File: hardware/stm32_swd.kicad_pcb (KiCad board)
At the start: 2 copper layers, 35 parts, among them J5 SWD_SWD, J6 SWD_SWD, U6 STM32F103C8T6_rect, U7 SWD, U8 AMS1117-3.3, U9 USBLC6-2SC6_SOT23-6, Y1 O_8M

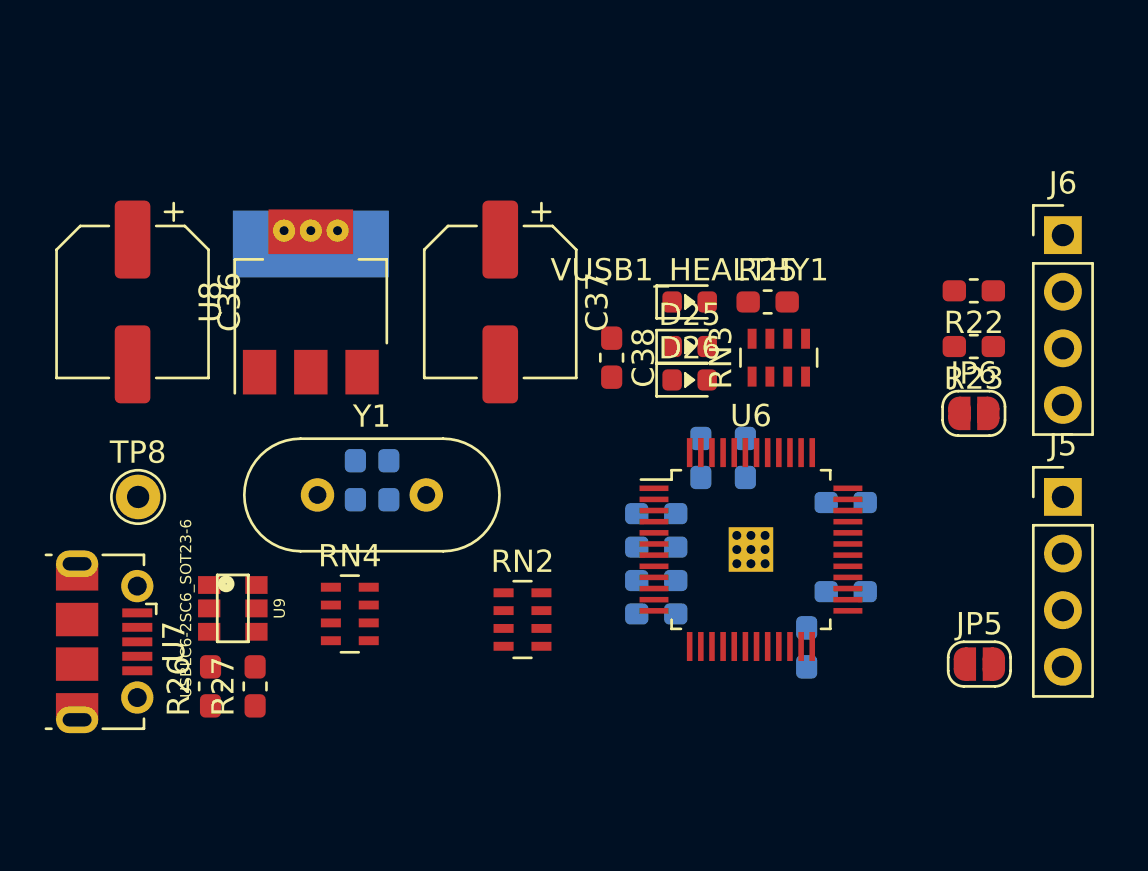
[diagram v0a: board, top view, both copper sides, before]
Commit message: update route,
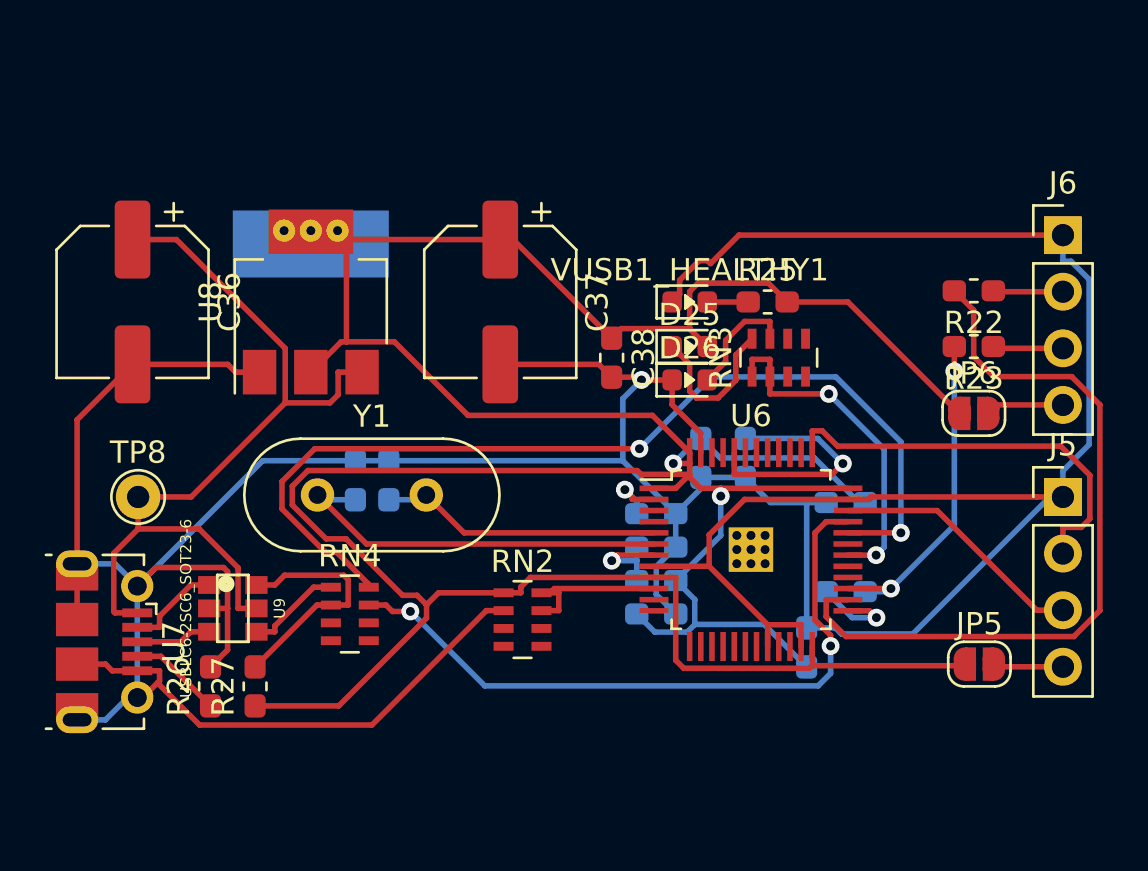
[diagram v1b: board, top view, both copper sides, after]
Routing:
- net GND: track 0.00 -> 200.6 mm, vias 0 -> 1
- net Vstm32_stlink: track 0.00 -> 166.6 mm, vias 0 -> 2
- net /USB_N: track 0.00 -> 44.0 mm, vias 0 -> 2
- net Vusb_1: track 0.00 -> 38.8 mm
- net /T_JTCK: track 0.00 -> 34.0 mm
- net /USB_P: track 0.00 -> 30.7 mm, vias 0 -> 2
- net /SWCLK: track 0.00 -> 18.8 mm
- net Net-(C29-Pad2): track 0.00 -> 17.8 mm
- net /LED_STLINK: track 0.00 -> 15.4 mm, vias 0 -> 2
- net /T_JTMS: track 0.00 -> 15.2 mm, vias 0 -> 2
- net Net-(C30-Pad2): track 0.00 -> 12.7 mm
- net /SWDIO: track 0.00 -> 11.5 mm
- net Net-(R20-Pad2): track 0.00 -> 10.9 mm, vias 0 -> 1
- net Net-(R27-Pad2): track 0.00 -> 10.8 mm
- net Net-(RN2-Pad7): track 0.00 -> 7.09 mm
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
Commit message: update ws2812,
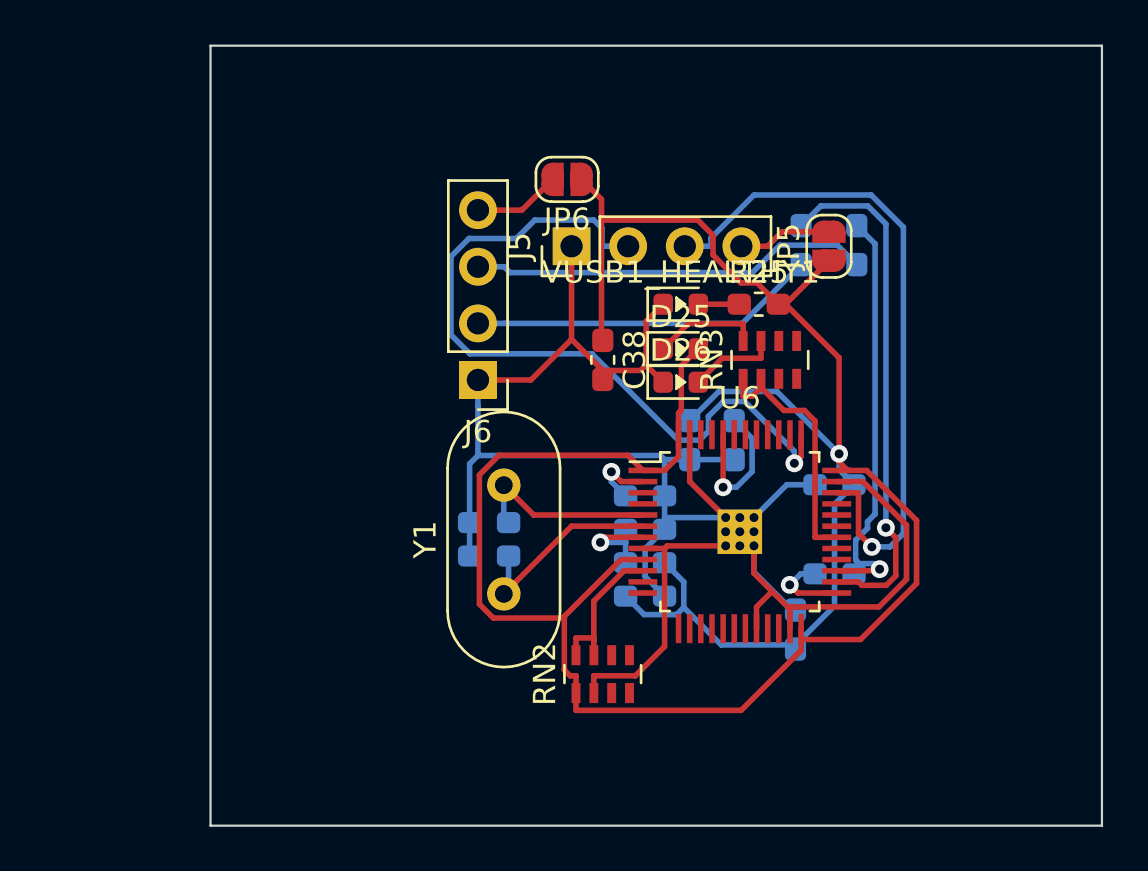
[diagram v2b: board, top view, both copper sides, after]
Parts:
- removed C36, C37: CP100uf,16V, Capacitor_SMD:CP_Elec_6.3x5.3
- removed R26: R104,0603, Resistor_SMD:R_0603_1608Metric_Pad1.05x0.95mm_HandSolder
- removed R27: R152,0603, Resistor_SMD:R_0603_1608Metric_Pad1.05x0.95mm_HandSolder
- removed RN4: RN_221,0603, Resistor_SMD:R_Array_Concave_4x0603
- removed TP8: TP_VUSB1, TestPoint:TestPoint_THTPad_D2.0mm_Drill1.0mm
- removed U7: SWD, footprint-lib:USB_Micro-B_Molex-105017-0001
- removed U8: AMS1117-3.3, footprint-lib:AMS1117_SOT-223
- removed U9: USBLC6-2SC6_SOT23-6, footprint-lib:USBLC6-2SC6_SOT23-6
- R22, R23: moved to B.Cu
- moved J6 27.0 mm to (42.0, 25.0), turned to 180 degrees
- moved J5 24.8 mm to (46.2, 19.0), turned to 90 degrees
- moved JP6 21.1 mm to (46.0, 16.0), turned to 180 degrees
- moved JP5 19.9 mm to (57.8, 19.0), turned to 90 degrees
- moved Y1 9.47 mm to (43.2, 34.6), turned to 90 degrees
- moved R22 8.02 mm to (56.5, 18.9), turned to 90 degrees
- moved R23 6.95 mm to (59.0, 18.9), turned to 90 degrees
- moved C29 6.90 mm to (42.5, 32.9), turned to 0 degrees
- moved C30 4.88 mm to (42.5, 31.4), turned to 0 degrees
- moved RN2 4.35 mm to (47.6, 38.2), turned to 90 degrees
- moved C31 0.94 mm to (51.5, 27.7)
- moved C32 0.94 mm to (49.5, 31.7)
- moved C34 0.94 mm to (58.0, 29.7)
- moved R19 0.94 mm to (49.5, 30.2)
- moved R20 0.94 mm to (53.5, 27.7)
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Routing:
- net GND: track 200.6 -> 94.7 mm, vias 1 -> 0
- net Vstm32_stlink: track 166.6 -> 118.9 mm, vias 2 -> 1
- net /USB_N: track 44.0 -> 0.00 mm, vias 2 -> 0
- net Vusb_1: track 38.8 -> 0.00 mm
- net /USB_P: track 30.7 -> 0.00 mm, vias 2 -> 0
- net /SWDIO: track 11.5 -> 30.6 mm, vias 0 -> 1
- net /SWCLK: track 18.8 -> 34.5 mm, vias 0 -> 1
- net /D_SWDIO: track 3.16 -> 18.0 mm
- net /D_SWCLK: track 3.14 -> 15.6 mm
- net Net-(R27-Pad2): track 10.8 -> 0.00 mm
- net /T_JTCK: track 34.0 -> 23.4 mm, vias 0 -> 1
- net Net-(C29-Pad2): track 17.8 -> 9.29 mm
- net Net-(R20-Pad2): track 10.9 -> 6.57 mm
- net Net-(RN4-Pad1): track 4.32 -> 0.00 mm
- net Net-(U7-Pad2): track 4.31 -> 0.00 mm
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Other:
- board outline added: 40 x 35 mm
